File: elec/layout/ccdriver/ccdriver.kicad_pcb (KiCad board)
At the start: 2 copper layers, 25.4 x 14.8 mm, 31 parts, among them U1 ?, U2 ?, U3 ?, U4 ?, U5 ?, U6 ?, U7 ?

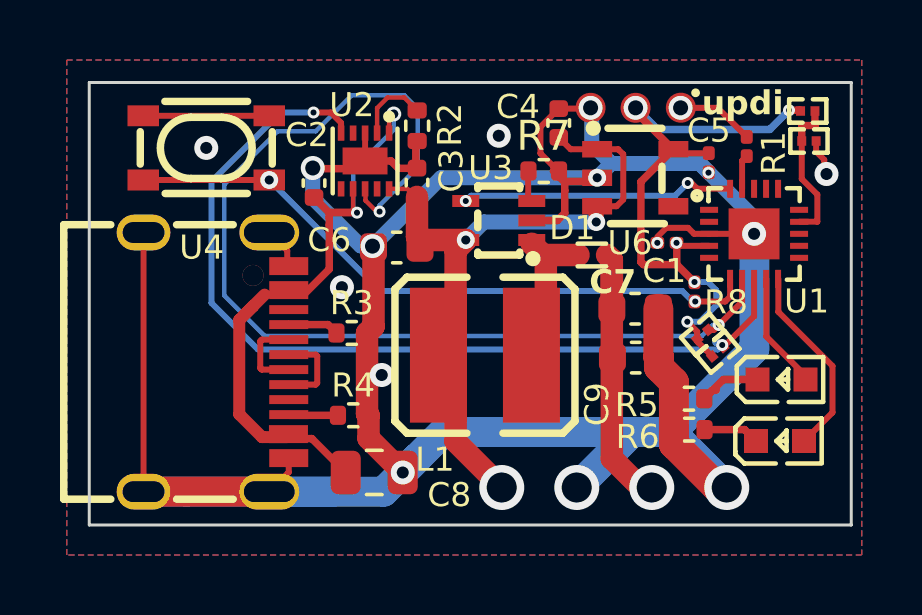
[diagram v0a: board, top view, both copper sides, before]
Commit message: new step models
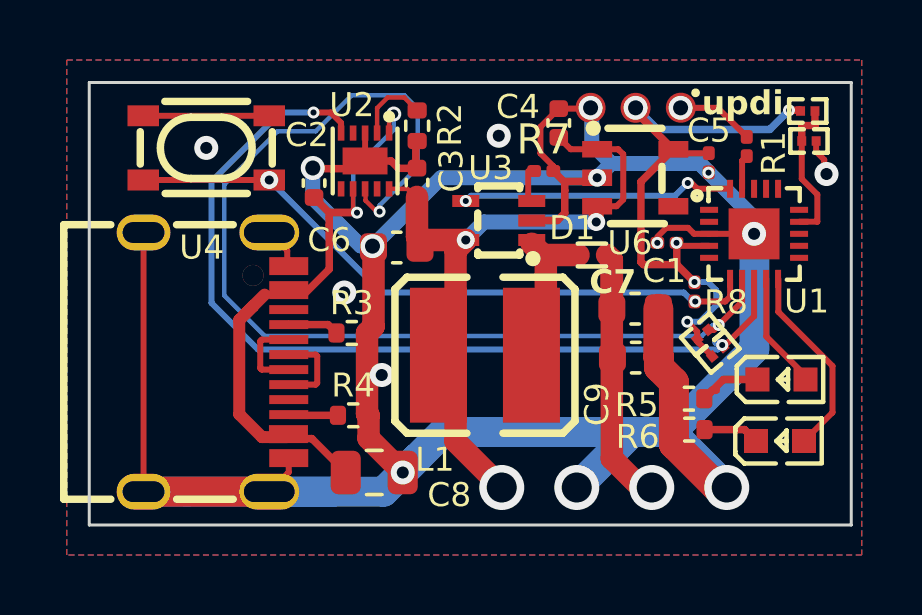
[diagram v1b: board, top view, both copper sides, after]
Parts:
- R7: value 62.5mW Thick Film Resistors 50V ±1% 300mΩ 0402 Chip Resistor - Surface Mount ROHS -> 100mW 300mΩ Chip Splitter 0ppm/℃~+300ppm/℃ ±1% 0201 Current Sense Resistors / Shunt Resistors ROHS; footprint lib:R0402 -> lib:R0201
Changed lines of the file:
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@@
 		)
 	)
-	(footprint "lib:R0402"
+	(footprint "lib:R0201"
 		(layer "F.Cu")
 		(at 184.4 114.2)
-		(descr "Resistor SMD 0402 (1005 Metric), square (rectangular) end terminal, IPC_7351 nominal, (Body size source: IPC-SM-782 page 72, https://www.pcb-3d.com/wordpress/wp-content/uploads/ipc-sm-782a_amendment_1_and_2.pdf), generated with kicad-footprint-generator")
+		(descr "Resistor SMD 0201 (0603 Metric), square (rectangular) end terminal, IPC_7351 nominal, (Body size source: https://www.vishay.com/docs/20052/crcw0201e3.pdf), generated with kicad-footprint-generator")
 		(tags "resistor")
 		(property "Reference" "R7"
-			(at 0 -1.17 0)
+			(at 0 -1.05 0)
 			(layer "F.SilkS")
 			(effects
@@
 			)
 		)
-		(property "Value" "62.5mW Thick Film Resistors 50V ±1% 300mΩ 0402  Chip Resistor - Surface Mount ROHS"
-			(at 0 1.17 0)
+		(property "Value" "100mW 300mΩ Chip Splitter 0ppm/℃~+300ppm/℃ ±1% 0201  Current Sense Resistors / Shunt Resistors ROHS"
+			(at 0 1.05 0)
 			(layer "F.Fab")
 			(effects
@@
 		(attr smd)
 		(fp_line
-			(start -0.153641 -0.38)
-			(end 0.153641 -0.38)
-			(stroke
-				(width 0.12)
-				(type solid)
-			)
-			(layer "F.SilkS")
-		)
-		(fp_line
-			(start -0.153641 0.38)
-			(end 0.153641 0.38)
-			(stroke
-				(width 0.12)
-				(type solid)
-			)
-			(layer "F.SilkS")
-		)
-		(fp_line
-			(start -0.93 -0.47)
-			(end 0.93 -0.47)
+			(start -0.7 -0.35)
+			(end 0.7 -0.35)
 			(stroke
 				(width 0.05)
@@
 		)
 		(fp_line
-			(start -0.93 0.47)
-			(end -0.93 -0.47)
+			(start -0.7 0.35)
+			(end -0.7 -0.35)
 			(stroke
 				(width 0.05)
@@
 		)
 		(fp_line
-			(start 0.93 -0.47)
-			(end 0.93 0.47)
+			(start 0.7 -0.35)
+			(end 0.7 0.35)
 			(stroke
 				(width 0.05)
@@
 		)
 		(fp_line
-			(start 0.93 0.47)
-			(end -0.93 0.47)
+			(start 0.7 0.35)
+			(end -0.7 0.35)
 			(stroke
 				(width 0.05)
@@
 		)
 		(fp_line
-			(start -0.525 -0.27)
-			(end 0.525 -0.27)
+			(start -0.3 -0.15)
+			(end 0.3 -0.15)
 			(stroke
 				(width 0.1)
@@
 		)
 		(fp_line
-			(start -0.525 0.27)
-			(end -0.525 -0.27)
+			(start -0.3 0.15)
+			(end -0.3 -0.15)
 			(stroke
 				(width 0.1)
@@
 		)
 		(fp_line
-			(start 0.525 -0.27)
-			(end 0.525 0.27)
+			(start 0.3 -0.15)
+			(end 0.3 0.15)
 			(stroke
 				(width 0.1)
@@
 		)
 		(fp_line
-			(start 0.525 0.27)
-			(end -0.525 0.27)
+			(start 0.3 0.15)
+			(end -0.3 0.15)
 			(stroke
 				(width 0.1)
@@
 		)
 		(fp_text user "${REFERENCE}"
-			(at 0 0 0)
+			(at 0 -0.68 0)
 			(layer "F.Fab")
 			(effects
 				(font
-					(size 0.26 0.26)
+					(size 0.25 0.25)
 					(thickness 0.04)
 				)
 			)
 		)
+		(pad "" smd roundrect
+			(at -0.345 0)
+			(size 0.318 0.36)
+			(layers "F.Paste")
+			(roundrect_rratio 0.25)
+		)
+		(pad "" smd roundrect
+			(at 0.345 0)
+			(size 0.318 0.36)
+			(layers "F.Paste")
+			(roundrect_rratio 0.25)
+		)
 		(pad "1" smd roundrect
-			(at -0.51 0)
-			(size 0.54 0.64)
-			(layers "F.Cu" "F.Paste" "F.Mask")
+			(at -0.32 0)
+			(size 0.46 0.4)
+			(layers "F.Cu" "F.Mask")
 			(roundrect_rratio 0.25)
 			(net 18 "fb")
@@
 		)
 		(pad "2" smd roundrect
-			(at 0.51 0)
-			(size 0.54 0.64)
-			(layers "F.Cu" "F.Paste" "F.Mask")
+			(at 0.32 0)
+			(size 0.46 0.4)
+			(layers "F.Cu" "F.Mask")
 			(roundrect_rratio 0.25)
 			(net 36 "gnd")
 			(pintype "stereo")
 		)
-		(model "${KICAD6_3DMODEL_DIR}/Resistor_SMD.3dshapes/R_0402_1005Metric.wrl"
+		(model "${KICAD6_3DMODEL_DIR}/Resistor_SMD.3dshapes/R_0201_0603Metric.wrl"
 			(offset
 				(xyz 0 0 0)
@@
 			(pintype "stereo")
 		)
-		(model "/home/lucy/atopile_projects/uv-lamp/build/footprints/footprints.3dshapes/R0201_L0.6-W0.3-H0.3.step"
+		(model "/home/lucy/Documents/atopile/uv-lamp/elec/footprints/footprints.3dshapes/R0201_L0.6-W0.3-H0.3.wrl"
 			(offset
 				(xyz 0 -0 0)
@@
 			(pintype "stereo")
 		)
-		(model "/home/lucy/atopile_projects/uv-lamp/build/footprints/footprints.3dshapes/R0201_L0.6-W0.3-H0.3.step"
+		(model "/home/lucy/Documents/atopile/uv-lamp/elec/footprints/footprints.3dshapes/R0201_L0.6-W0.3-H0.3.step"
 			(offset
 				(xyz 0 -0 0)
@@
 			(pintype "stereo")
 		)
-		(model "/home/lucy/atopile_projects/uv-lamp/build/footprints/footprints.3dshapes/R0201_L0.6-W0.3-H0.3.step"
+		(model "/home/lucy/Documents/atopile/uv-lamp/elec/footprints/footprints.3dshapes/R0201_L0.6-W0.3-H0.3.wrl"
 			(offset
 				(xyz 0 -0 0)
@@
 			(pintype "stereo")
 		)
-		(model "/home/lucy/atopile_projects/uv-lamp/build/footprints/footprints.3dshapes/R0201_L0.6-W0.3-H0.3.step"
+		(model "/home/lucy/Documents/atopile/uv-lamp/elec/footprints/footprints.3dshapes/R0201_L0.6-W0.3-H0.3.wrl"
 			(offset
-				(xyz -0 -0 0)
+				(xyz 0 0 0)
 			)
 			(scale
@@
 	)
 	(segment
-		(start 189.45 118.55)
-		(end 189.367893 118.55)
+		(start 189.367893 118.55)
+		(end 189.067893 118.25)
 		(width 0.2)
 		(layer "B.Cu")
@@
 	)
 	(segment
-		(start 189.367893 118.55)
-		(end 189.017893 118.2)
+		(start 179 118.25)
+		(end 175.25 114.5)
 		(width 0.2)
 		(layer "B.Cu")
@@
 	)
 	(segment
-		(start 189.017893 118.2)
-		(end 178.95 118.2)
+		(start 189.067893 118.25)
+		(end 179 118.25)
 		(width 0.2)
 		(layer "B.Cu")
@@
 	)
 	(segment
-		(start 178.95 118.2)
-		(end 175.25 114.5)
+		(start 189.45 118.55)
+		(end 189.367893 118.55)
 		(width 0.2)
 		(layer "B.Cu")
@@
 	)
 	(via
+		(at 177.75 118.25)
+		(size 0.8)
+		(drill 0.4)
+		(layers "F.Cu" "B.Cu")
+		(net 36)
+	)
+	(via
 		(at 189.891149 114.254269)
 		(size 0.4)
@@
 		(net 36)
 	)
-	(via
-		(at 177.672653 118.072653)
-		(size 0.8)
-		(drill 0.4)
-		(layers "F.Cu" "B.Cu")
-		(net 36)
-	)
